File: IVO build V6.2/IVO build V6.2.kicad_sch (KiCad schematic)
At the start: 15 parts, among them U1 L7805, U2 1EDI60I12AF, U3 MGJ1D121505MPC-R7

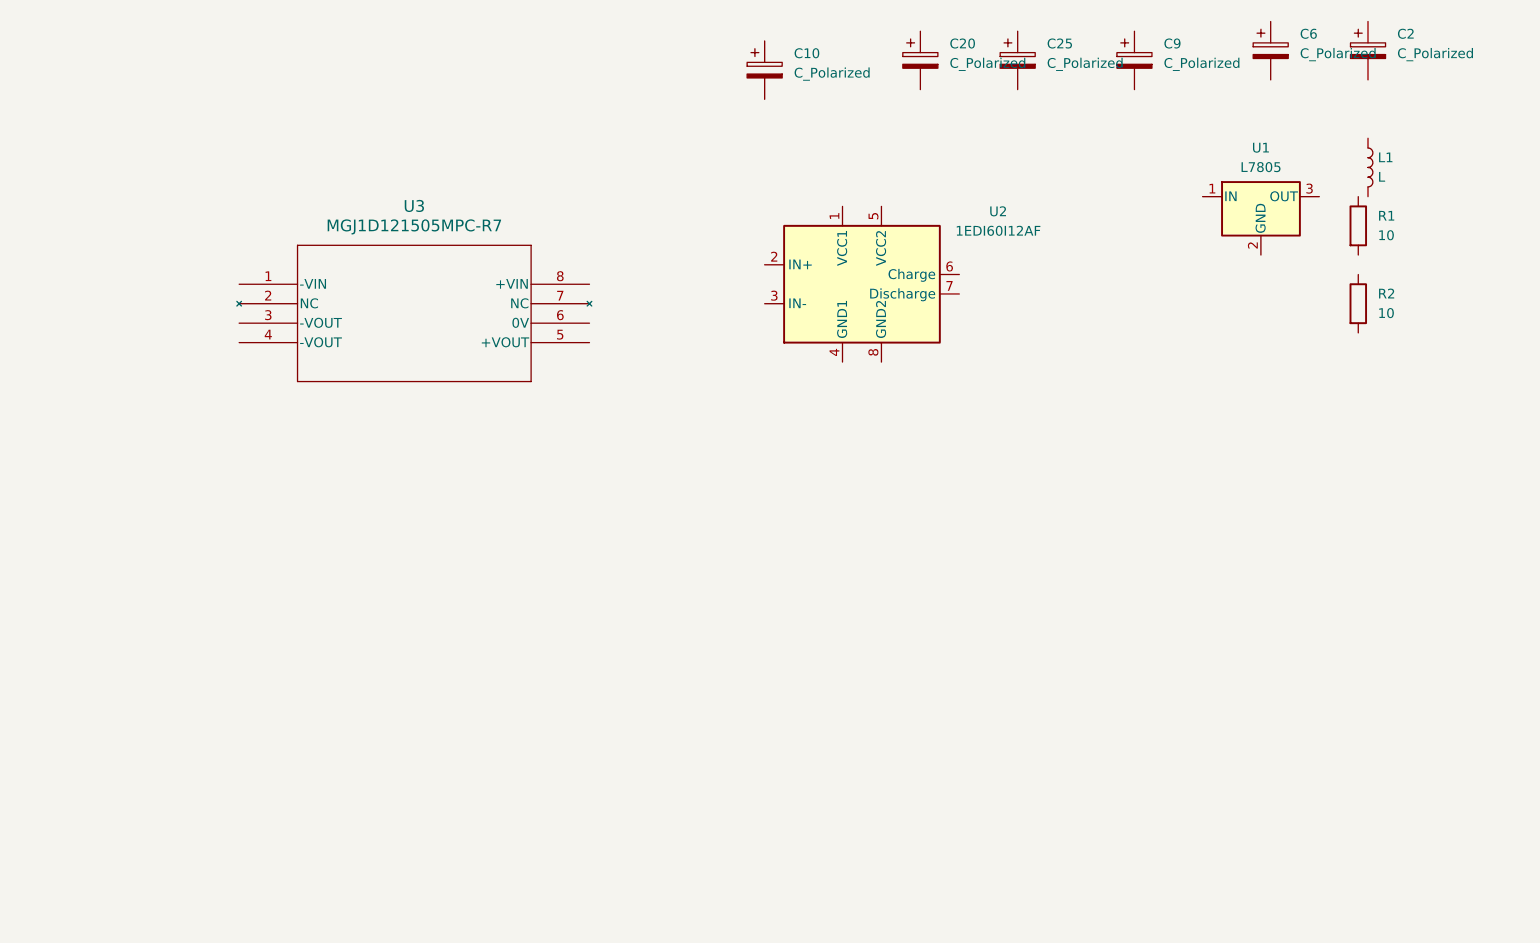
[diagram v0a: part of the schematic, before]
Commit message: Updated schematic
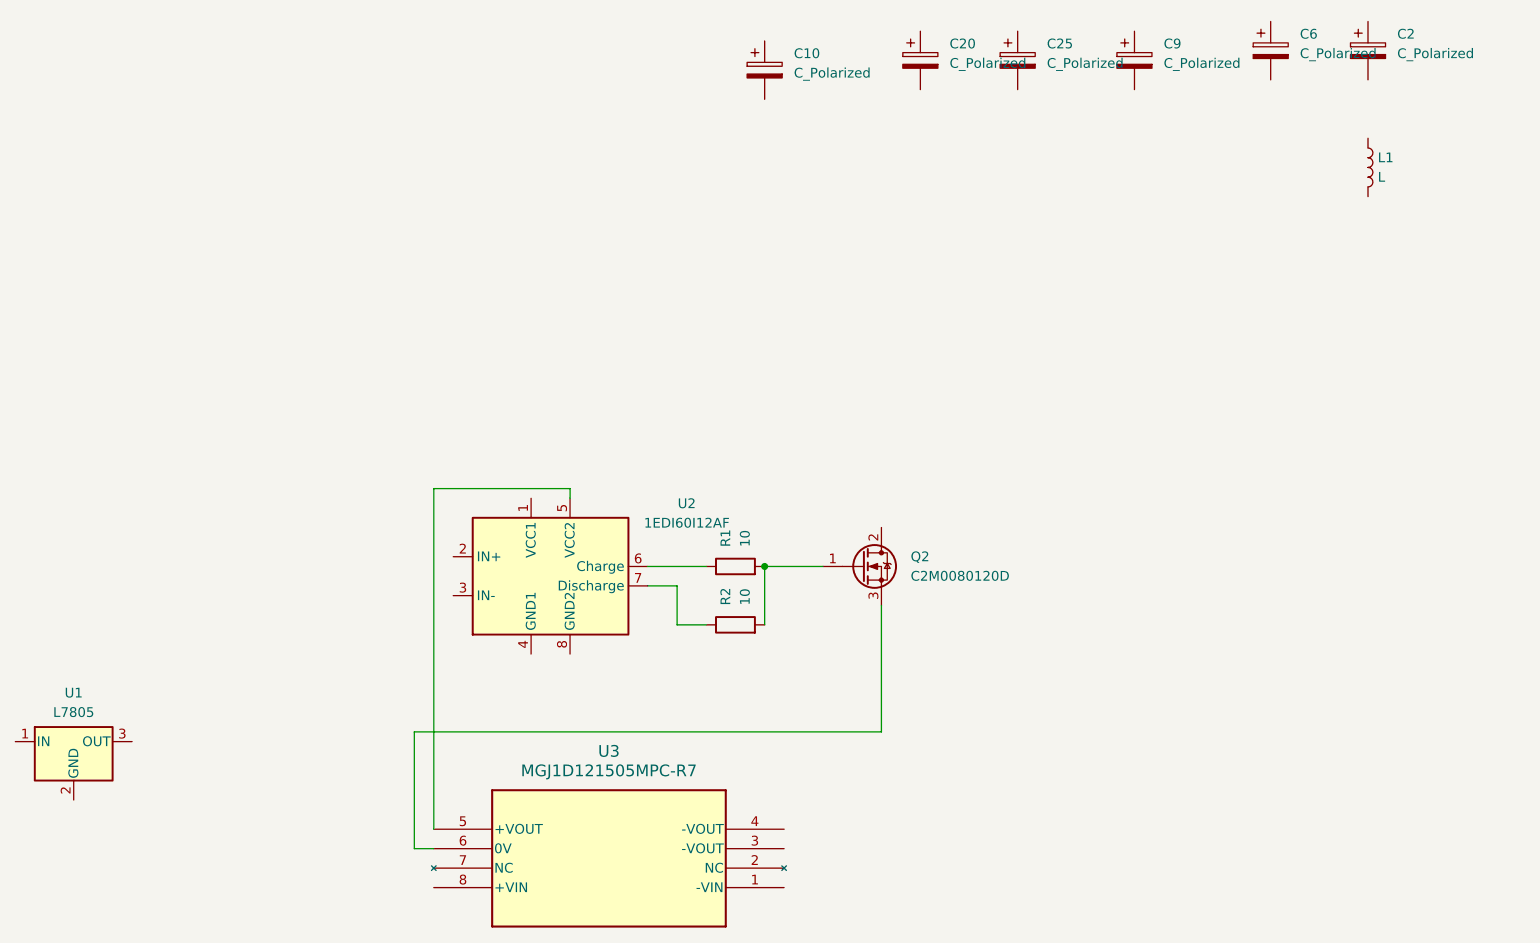
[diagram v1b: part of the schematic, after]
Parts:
- added Q2: C2M0080120D, Package_TO_SOT_THT:TO-247-3_Vertical, symbol Transistor_FET:C2M0080120D
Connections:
- net at U3.5 (+VOUT): now also U2.5 (VCC2)
- net at U3.6 (0V): now also Q2.3 (S)
- net at R2.1: now also U2.7 (Discharge)
- net at R2.2: now also R1.2, Q2.1 (G)
- net at R1.1: now also U2.6 (Charge)
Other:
- moved on the sheet: R1, R2, U1, U2
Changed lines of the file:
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@@
     (rev "V1.0")
+  )
+  (junction (at 195.58 101.6) (diameter 0) (color 0 0 0 0)
+  )
+  (wire (pts (xy 170.18 91.44) (xy 170.18 92.71))
+    (stroke (width 0) (type default))
+  )
+  (wire (pts (xy 152.4 135.89) (xy 152.4 91.44))
+    (stroke (width 0) (type default))
+  )
+  (wire (pts (xy 195.58 101.6) (xy 195.58 109.22))
+    (stroke (width 0) (type default))
+  )
+  (wire (pts (xy 184.15 109.22) (xy 187.96 109.22))
+    (stroke (width 0) (type default))
+  )
+  (wire (pts (xy 180.34 101.6) (xy 187.96 101.6))
+    (stroke (width 0) (type default))
+  )
+  (wire (pts (xy 195.58 101.6) (xy 203.2 101.6))
+    (stroke (width 0) (type default))
+  )
+  (wire (pts (xy 180.34 104.14) (xy 184.15 104.14))
+    (stroke (width 0) (type default))
+  )
+  (wire (pts (xy 149.86 138.43) (xy 149.86 123.19))
+    (stroke (width 0) (type default))
+  )
+  (wire (pts (xy 149.86 123.19) (xy 210.82 123.19))
+    (stroke (width 0) (type default))
+  )
+  (wire (pts (xy 152.4 91.44) (xy 170.18 91.44))
+    (stroke (width 0) (type default))
+  )
+  (wire (pts (xy 152.4 138.43) (xy 149.86 138.43))
+    (stroke (width 0) (type default))
+  )
+  (wire (pts (xy 210.82 123.19) (xy 210.82 106.68))
+    (stroke (width 0) (type default))
+  )
+  (wire (pts (xy 184.15 104.14) (xy 184.15 109.22))
+    (stroke (width 0) (type default))
   )
   (text_box "C10\nC2,C6 (both for 2 caps, sorry)\nC7\nC8\nC9\nC25\nC20\nC3  (c6 c2 and between pin 5 and 8 of U1)\nL1\nGDS / Q1\nR1,R2\nU1 (smd not labeled sorry)\nU3\nbottom square\n"
@@
     (effects (font (size 1.27 1.27)) (justify left top))
   )
-  (symbol (lib_id "Regulator_Linear:L7805") (at 260.35 53.34 0) (unit 1)
-    (exclude_from_sim no) (in_bom yes) (on_board yes) (dnp no) (fields_autoplaced)
-    (property "Reference" "U1" (at 260.35 46.99 0)
+  (symbol (lib_id "Regulator_Linear:L7805") (at 105.41 124.46 0) (unit 1)
+    (exclude_from_sim no) (in_bom yes) (on_board yes) (dnp no) (fields_autoplaced)
+    (property "Reference" "U1" (at 105.41 118.11 0)
       (effects (font (size 1.27 1.27)))
     )
-    (property "Value" "L7805" (at 260.35 49.53 0)
+    (property "Value" "L7805" (at 105.41 120.65 0)
       (effects (font (size 1.27 1.27)))
     )
-    (property "Footprint" "" (at 260.985 57.15 0)
+    (property "Footprint" "" (at 106.045 128.27 0)
       (effects (font (size 1.27 1.27) italic) (justify left) hide)
     )
-    (property "Datasheet" "http://www.st.com/content/ccc/resource/technical/document/datasheet/41/4f/b3/b0/12/d4/47/88/CD00000444.pdf/files/CD00000444.pdf/jcr:content/translations/en.CD00000444.pdf" (at 260.35 54.61 0)
-      (effects (font (size 1.27 1.27)) hide)
-    )
-    (property "Description" "Positive 1.5A 35V Linear Regulator, Fixed Output 5V, TO-220/TO-263/TO-252" (at 260.35 53.34 0)
+    (property "Datasheet" "http://www.st.com/content/ccc/resource/technical/document/datasheet/41/4f/b3/b0/12/d4/47/88/CD00000444.pdf/files/CD00000444.pdf/jcr:content/translations/en.CD00000444.pdf" (at 105.41 125.73 0)
+      (effects (font (size 1.27 1.27)) hide)
+    )
+    (property "Description" "Positive 1.5A 35V Linear Regulator, Fixed Output 5V, TO-220/TO-263/TO-252" (at 105.41 124.46 0)
       (effects (font (size 1.27 1.27)) hide)
     )
@@
     )
   )
-  (symbol (lib_id "2023-11-16_09-14-49:MGJ1D121505MPC-R7") (at 127 64.77 0) (unit 1)
-    (exclude_from_sim no) (in_bom yes) (on_board yes) (dnp no) (fields_autoplaced)
-    (property "Reference" "U3" (at 149.86 54.61 0)
+  (symbol (lib_id "2023-11-16_09-14-49:MGJ1D121505MPC-R7") (at 198.12 143.51 180) (unit 1)
+    (exclude_from_sim no) (in_bom yes) (on_board yes) (dnp no) (fields_autoplaced)
+    (property "Reference" "U3" (at 175.26 125.73 0)
       (effects (font (size 1.524 1.524)))
     )
-    (property "Value" "MGJ1D121505MPC-R7" (at 149.86 57.15 0)
+    (property "Value" "MGJ1D121505MPC-R7" (at 175.26 128.27 0)
       (effects (font (size 1.524 1.524)))
     )
-    (property "Footprint" "MGJ1_MUR" (at 127 64.77 0)
+    (property "Footprint" "MGJ1_MUR" (at 198.12 143.51 0)
       (effects (font (size 1.27 1.27) italic) hide)
     )
-    (property "Datasheet" "MGJ1D121505MPC-R7" (at 127 64.77 0)
+    (property "Datasheet" "MGJ1D121505MPC-R7" (at 198.12 143.51 0)
       (effects (font (size 1.27 1.27) italic) hide)
     )
-    (property "Description" "" (at 127 64.77 0)
+    (property "Description" "" (at 198.12 143.51 0)
       (effects (font (size 1.27 1.27)) hide)
     )
@@
     )
   )
-  (symbol (lib_id "Device:R") (at 273.05 67.31 0) (unit 1)
-    (exclude_from_sim no) (in_bom yes) (on_board yes) (dnp no) (fields_autoplaced)
-    (property "Reference" "R2" (at 275.59 66.0399 0)
-      (effects (font (size 1.27 1.27)) (justify left))
-    )
-    (property "Value" "10" (at 275.59 68.5799 0)
-      (effects (font (size 1.27 1.27)) (justify left))
-    )
-    (property "Footprint" "" (at 271.272 67.31 90)
-      (effects (font (size 1.27 1.27)) hide)
-    )
-    (property "Datasheet" "~" (at 273.05 67.31 0)
-      (effects (font (size 1.27 1.27)) hide)
-    )
-    (property "Description" "Resistor" (at 273.05 67.31 0)
+  (symbol (lib_id "Transistor_FET:C2M0080120D") (at 208.28 101.6 0) (unit 1)
+    (exclude_from_sim no) (in_bom yes) (on_board yes) (dnp no) (fields_autoplaced)
+    (property "Reference" "Q2" (at 214.63 100.3299 0)
+      (effects (font (size 1.27 1.27)) (justify left))
+    )
+    (property "Value" "C2M0080120D" (at 214.63 102.8699 0)
+      (effects (font (size 1.27 1.27)) (justify left))
+    )
+    (property "Footprint" "Package_TO_SOT_THT:TO-247-3_Vertical" (at 208.28 101.6 0)
+      (effects (font (size 1.27 1.27) italic) hide)
+    )
+    (property "Datasheet" "https://www.wolfspeed.com/media/downloads/167/C2M0080120D.pdf" (at 208.28 101.6 0)
+      (effects (font (size 1.27 1.27)) (justify left) hide)
+    )
+    (property "Description" "36A Id, 1200V Vds, 80mOhm, N-Channel SiC MOSFET, TO-247" (at 208.28 101.6 0)
+      (effects (font (size 1.27 1.27)) hide)
+    )
+    (pin "2")
+    (pin "3")
+    (pin "1")
+    (instances
+      (project "IVO build V6.2"
+        (path "/b677c1c3-d122-4e96-b301-95dfb1fcc78b"
+          (reference "Q2") (unit 1)
+        )
+      )
+    )
+  )
+  (symbol (lib_id "Device:R") (at 191.77 109.22 90) (unit 1)
+    (exclude_from_sim no) (in_bom yes) (on_board yes) (dnp no) (fields_autoplaced)
+    (property "Reference" "R2" (at 190.4999 106.68 0)
+      (effects (font (size 1.27 1.27)) (justify left))
+    )
+    (property "Value" "10" (at 193.0399 106.68 0)
+      (effects (font (size 1.27 1.27)) (justify left))
+    )
+    (property "Footprint" "" (at 191.77 110.998 90)
+      (effects (font (size 1.27 1.27)) hide)
+    )
+    (property "Datasheet" "~" (at 191.77 109.22 0)
+      (effects (font (size 1.27 1.27)) hide)
+    )
+    (property "Description" "Resistor" (at 191.77 109.22 0)
       (effects (font (size 1.27 1.27)) hide)
     )
@@
     )
   )
-  (symbol (lib_id "Device:R") (at 273.05 57.15 0) (unit 1)
-    (exclude_from_sim no) (in_bom yes) (on_board yes) (dnp no) (fields_autoplaced)
-    (property "Reference" "R1" (at 275.59 55.8799 0)
-      (effects (font (size 1.27 1.27)) (justify left))
-    )
-    (property "Value" "10" (at 275.59 58.4199 0)
-      (effects (font (size 1.27 1.27)) (justify left))
-    )
-    (property "Footprint" "" (at 271.272 57.15 90)
-      (effects (font (size 1.27 1.27)) hide)
-    )
-    (property "Datasheet" "~" (at 273.05 57.15 0)
-      (effects (font (size 1.27 1.27)) hide)
-    )
-    (property "Description" "Resistor" (at 273.05 57.15 0)
+  (symbol (lib_id "Device:R") (at 191.77 101.6 90) (unit 1)
+    (exclude_from_sim no) (in_bom yes) (on_board yes) (dnp no) (fields_autoplaced)
+    (property "Reference" "R1" (at 190.4999 99.06 0)
+      (effects (font (size 1.27 1.27)) (justify left))
+    )
+    (property "Value" "10" (at 193.0399 99.06 0)
+      (effects (font (size 1.27 1.27)) (justify left))
+    )
+    (property "Footprint" "" (at 191.77 103.378 90)
+      (effects (font (size 1.27 1.27)) hide)
+    )
+    (property "Datasheet" "~" (at 191.77 101.6 0)
+      (effects (font (size 1.27 1.27)) hide)
+    )
+    (property "Description" "Resistor" (at 191.77 101.6 0)
       (effects (font (size 1.27 1.27)) hide)
     )
@@
     )
   )
-  (symbol (lib_id "Driver_FET:STGAP2SCM") (at 208.28 64.77 0) (unit 1)
-    (exclude_from_sim no) (in_bom yes) (on_board yes) (dnp no) (fields_autoplaced)
-    (property "Reference" "U2" (at 226.06 55.3018 0)
+  (symbol (lib_id "Driver_FET:STGAP2SCM") (at 167.64 102.87 0) (unit 1)
+    (exclude_from_sim no) (in_bom yes) (on_board yes) (dnp no) (fields_autoplaced)
+    (property "Reference" "U2" (at 185.42 93.4018 0)
       (effects (font (size 1.27 1.27)))
     )
-    (property "Value" "1EDI60I12AF" (at 226.06 57.8418 0)
+    (property "Value" "1EDI60I12AF" (at 185.42 95.9418 0)
       (effects (font (size 1.27 1.27)))
     )
-    (property "Footprint" "Package_SO:SOIC-8_3.9x4.9mm_P1.27mm" (at 208.28 95.25 0)
-      (effects (font (size 1.27 1.27)) hide)
-    )
-    (property "Datasheet" "https://www.st.com/resource/en/datasheet/stgap2s.pdf" (at 207.01 91.44 0)
-      (effects (font (size 1.27 1.27)) hide)
-    )
-    (property "Description" "Galvanically isolated 4 A single gate driver, Single Output, Miller Clamp, SOIC-8" (at 210.82 87.63 0)
-      (effects (font (size 1.27 1.27)) hide)
-    )
+    (property "Footprint" "Package_SO:SOIC-8_3.9x4.9mm_P1.27mm" (at 167.64 133.35 0)
+      (effects (font (size 1.27 1.27)) hide)
+    )
+    (property "Datasheet" "https://www.st.com/resource/en/datasheet/stgap2s.pdf" (at 166.37 129.54 0)
+      (effects (font (size 1.27 1.27)) hide)
+    )
+    (property "Description" "Galvanically isolated 4 A single gate driver, Single Output, Miller Clamp, SOIC-8" (at 170.18 125.73 0)
+      (effects (font (size 1.27 1.27)) hide)
+    )

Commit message: Updated schematic
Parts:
- U3: footprint MGJ1_MUR -> footprints:MGJ1_MUR
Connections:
- net at U1.1 (IN): now also L1.2, U3.8 (+VIN)
- net GND: now reaches U1.2 (GND)
- net GND: now also U2.4 (GND1)
- net at U1.3 (OUT): now also U2.1 (VCC1)
- net +12V: now reaches L1.1
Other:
- moved on the sheet: L1, Q2, R1, R2, U1, U2, U3

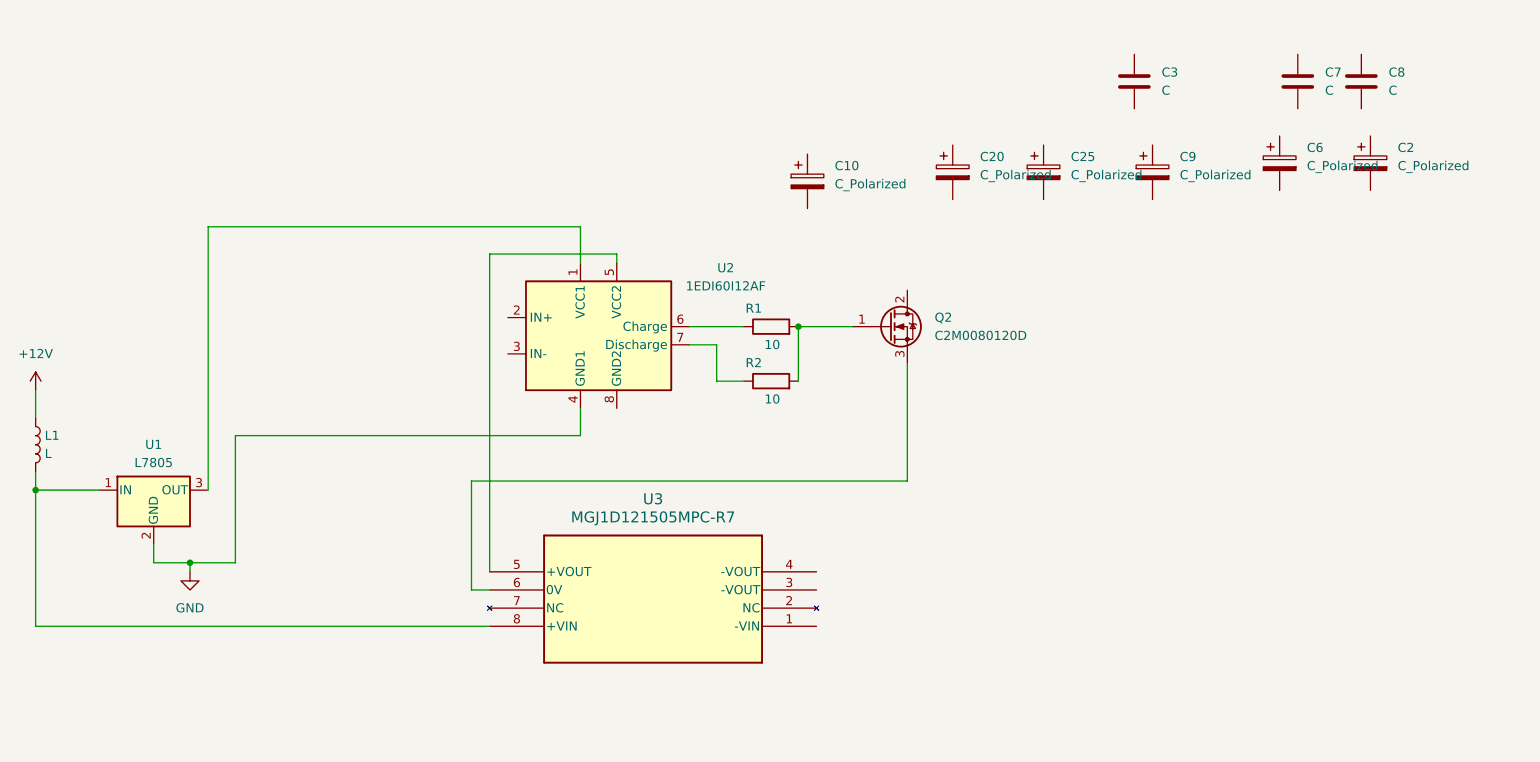
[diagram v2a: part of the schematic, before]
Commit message: Updated schematic
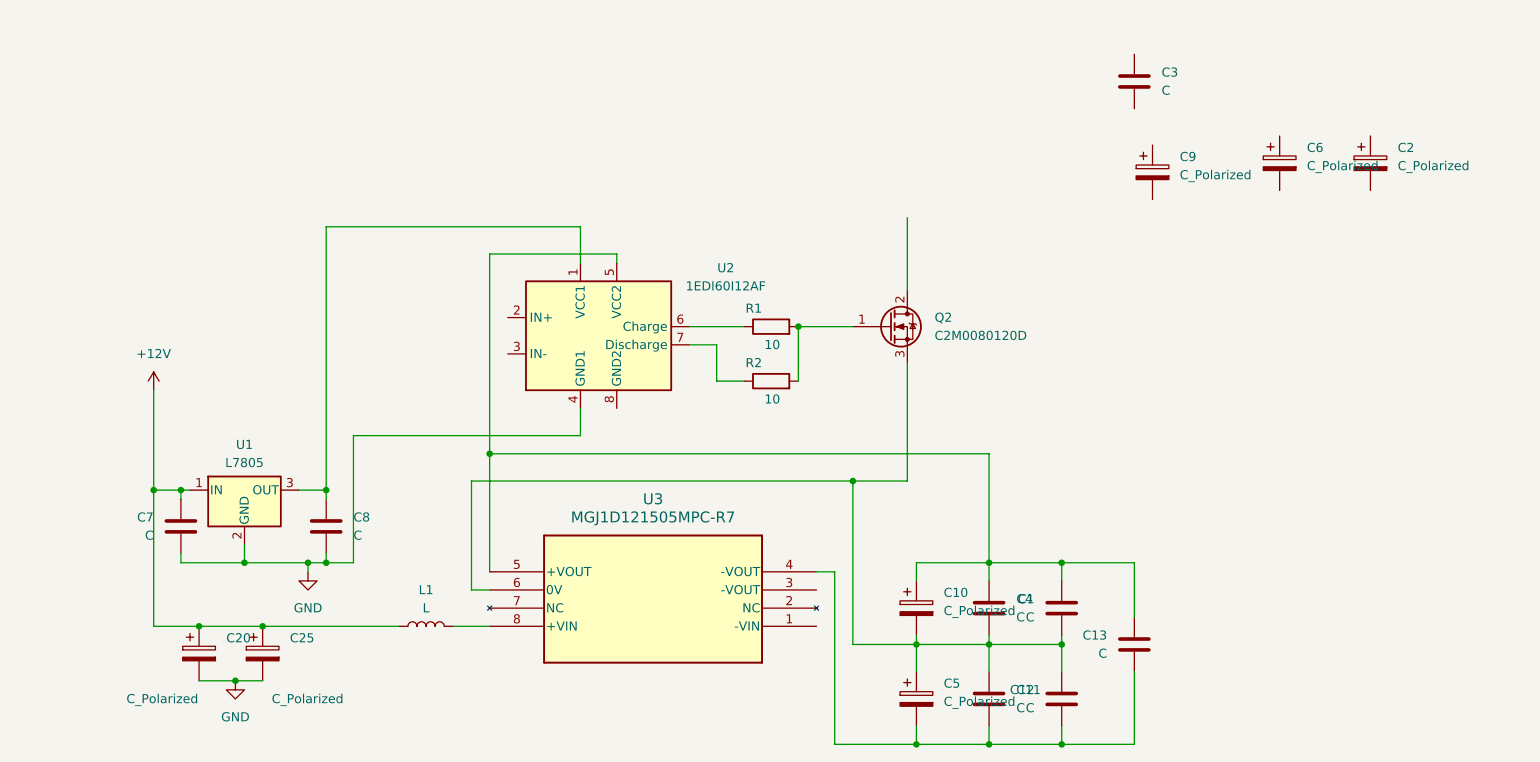
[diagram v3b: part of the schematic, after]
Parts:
- added C1, C11, C12, C13, C4: C, symbol Device:C
- added C5: C_Polarized, symbol Device:C_Polarized
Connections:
- net +12V: now also C20.1, C25.1, C7.1, U1.1 (IN)
- net GND: now also C20.2, C25.2, C7.2, C8.2
- net at L1.2, U3.8 (+VIN): no longer U1.1 (IN)
- net at U1.3 (OUT), U2.1 (VCC1): now also C8.1
- net at U3.4 (-VOUT): now also C11.2, C12.2, C13.2, C5.2
- net at U2.5 (VCC2), U3.5 (+VOUT): now also C10.1, C1.1, C13.1, C4.1
- net at Q2.3 (S), U3.6 (0V): now also C10.2, C1.2, C11.1, C12.1, C4.2, C5.1
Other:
- title: IVO driver board -> IVO driver board 6.2
- moved on the sheet: C10, C20, C25, C7, C8, U1
